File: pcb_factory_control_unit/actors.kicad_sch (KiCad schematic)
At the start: 79 parts, among them J17 Elevator, J18 Sorter, J19 Vacuum Pump, J20 Bus-Servo, J21 Cylinder Valve, J22 RoArm, J23 Conveyor, J24 Compressor, J25 Vacuum Valve, J26 Disturbance1, J27 Disturbance2, Q3 AO3400, Q4 AO3400, Q5 AO3400, Q6 AO3400, Q7 AO3400, Q8 AO3400, U10 TMC2209, U11 74AHCT125, U9 TMC2209

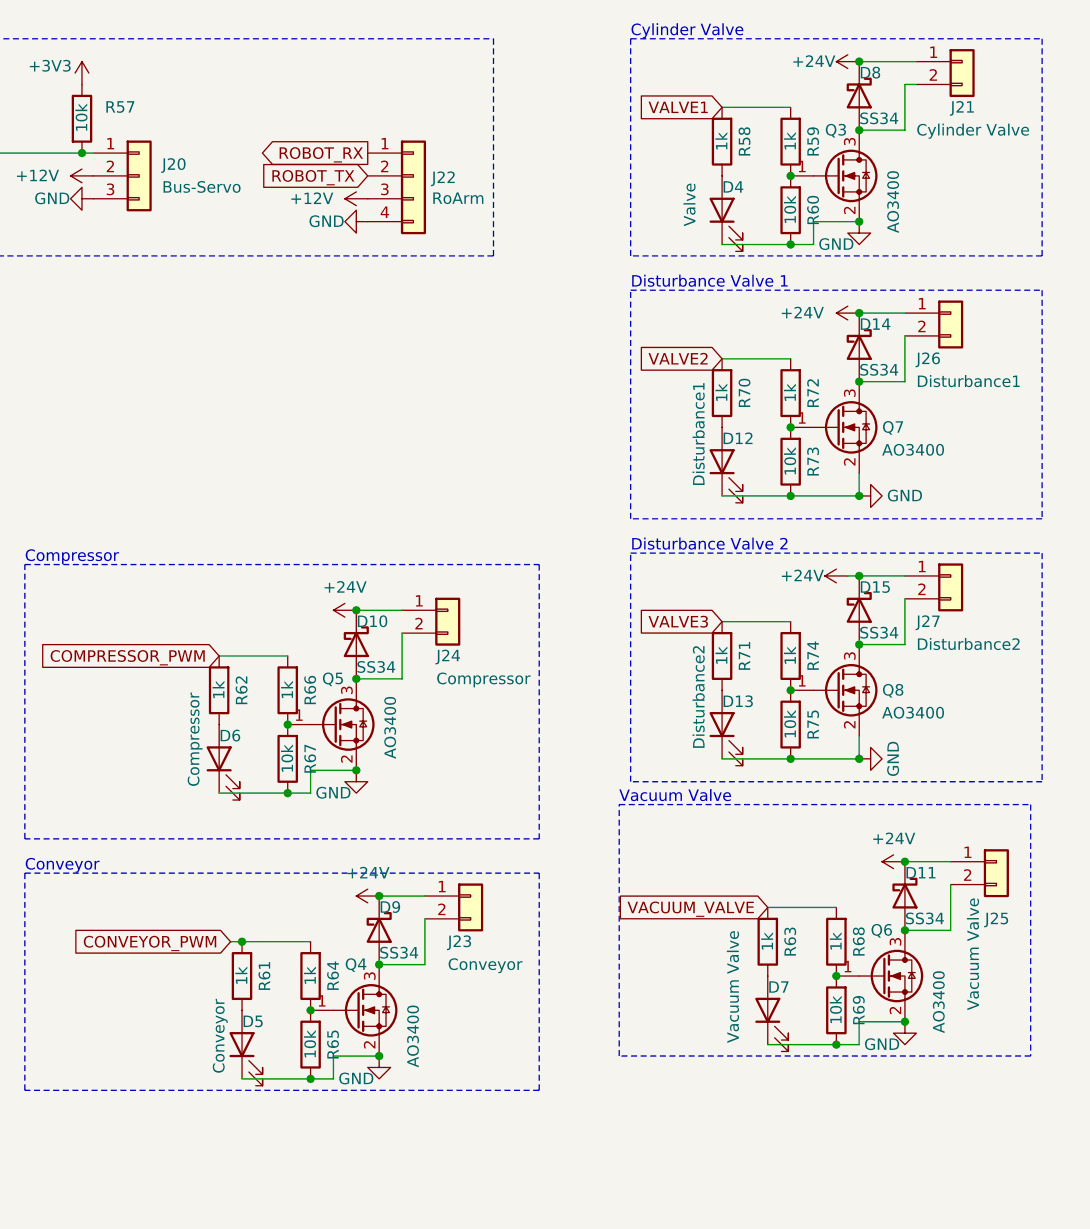
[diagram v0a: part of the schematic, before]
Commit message: FCB ready for review
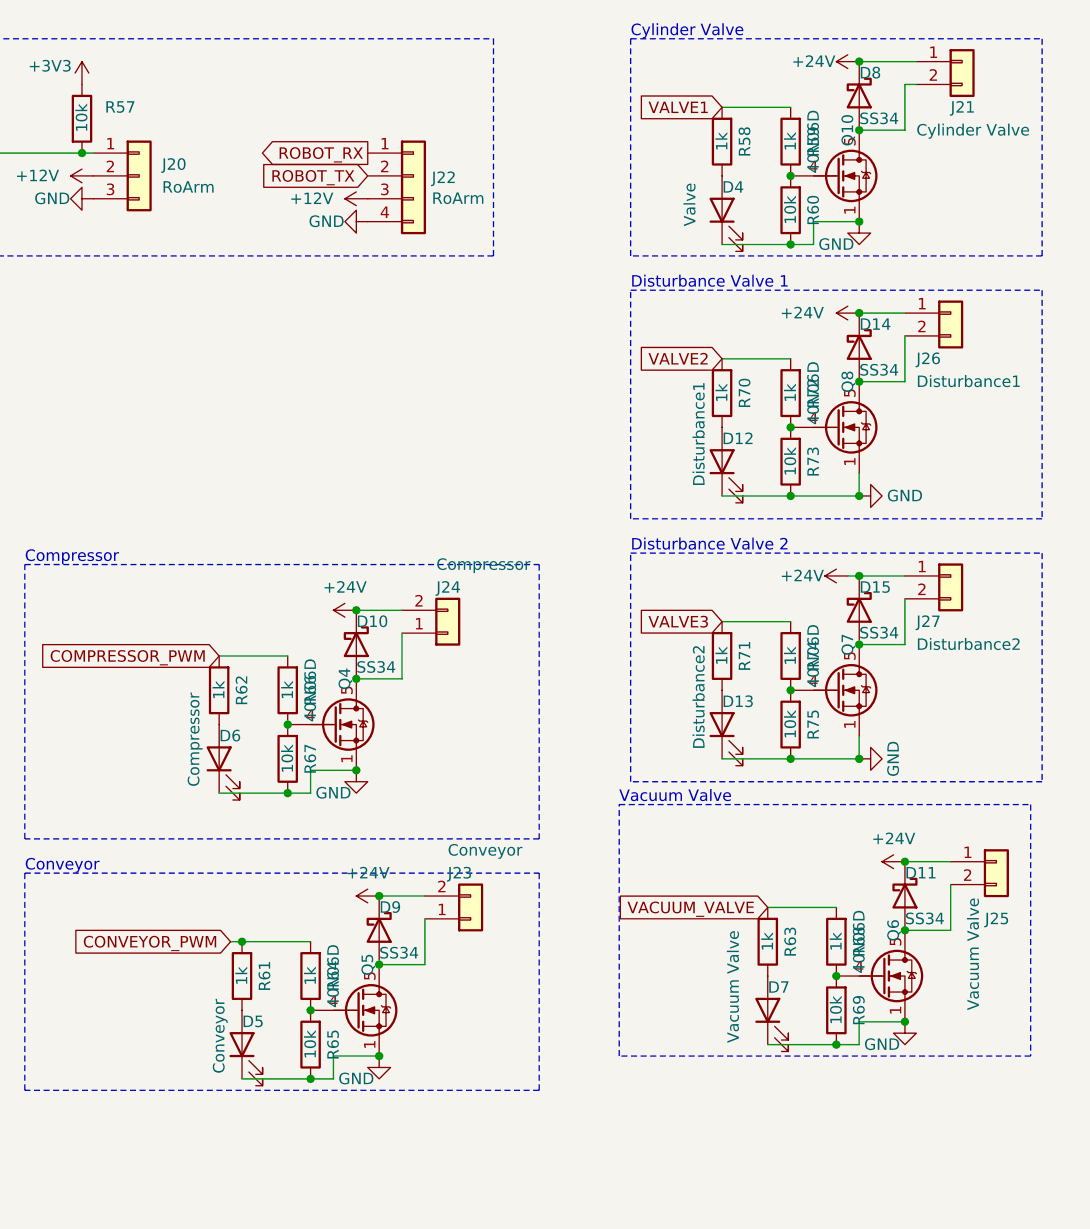
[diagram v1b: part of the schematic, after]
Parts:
- removed Q3, Q4, Q5, Q6, Q7, Q8: AO3400, Package_TO_SOT_SMD:SOT-23, symbol Transistor_FET:IRLML0030
- added Q10, Q4, Q5, Q6, Q7, Q8: 40N06D, Package_SON:VSON-8_3.3x3.3mm_P0.65mm_NexFET, symbol Transistor_FET:CSD18543Q3A
- J20: value Bus-Servo -> RoArm
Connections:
- net +24V: now also J23.2 (Pin_2), J24.2 (Pin_2); no longer J23.1 (Pin_1), J24.1 (Pin_1)
- net GND: now also Q10.1 (S), Q10.2 (S), Q10.3 (S), Q4.1 (S), Q4.2 (S), Q4.3 (S), Q5.1 (S), Q5.2 (S), Q5.3 (S), Q6.1 (S), Q6.2 (S), Q6.3 (S), Q7.1 (S), Q7.2 (S), Q7.3 (S), Q8.1 (S), Q8.2 (S), Q8.3 (S)
- net at R72.1, R73.2: now also Q8.4 (G)
- net at D15.2 (A), J27.2 (Pin_2): now also Q7.5 (D)
- net at D8.2 (A), J21.2 (Pin_2): now also Q10.5 (D)
- net at R74.1, R75.2: now also Q7.4 (G)
- net at R64.1, R65.2: now also Q5.4 (G)
- net at D9.2 (A): now also J23.1 (Pin_1), Q5.5 (D); no longer J23.2 (Pin_2)
- net at R66.1, R67.2: now also Q4.4 (G)
- net at D10.2 (A): now also J24.1 (Pin_1), Q4.5 (D); no longer J24.2 (Pin_2)
- net at R68.1, R69.2: now also Q6.4 (G)
- net at D14.2 (A), J26.2 (Pin_2): now also Q8.5 (D)
- net at D11.2 (A), J25.2 (Pin_2): now also Q6.5 (D)
- net at R59.1, R60.2: now also Q10.4 (G)
